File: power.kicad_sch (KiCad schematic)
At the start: 89 parts, among them Q1 PJE138K, Q2 PJE138K, Q3 SSM3J332R, Q4 PJE138K, Q5 SSM3J332R, Q6 PJE138K, Q7 SSM3J332R, U1 TLV70018_SC70, U4 TPS65150_HTSSOP, U5 MPQ7235GQBE, U6 TLV76701_WSON

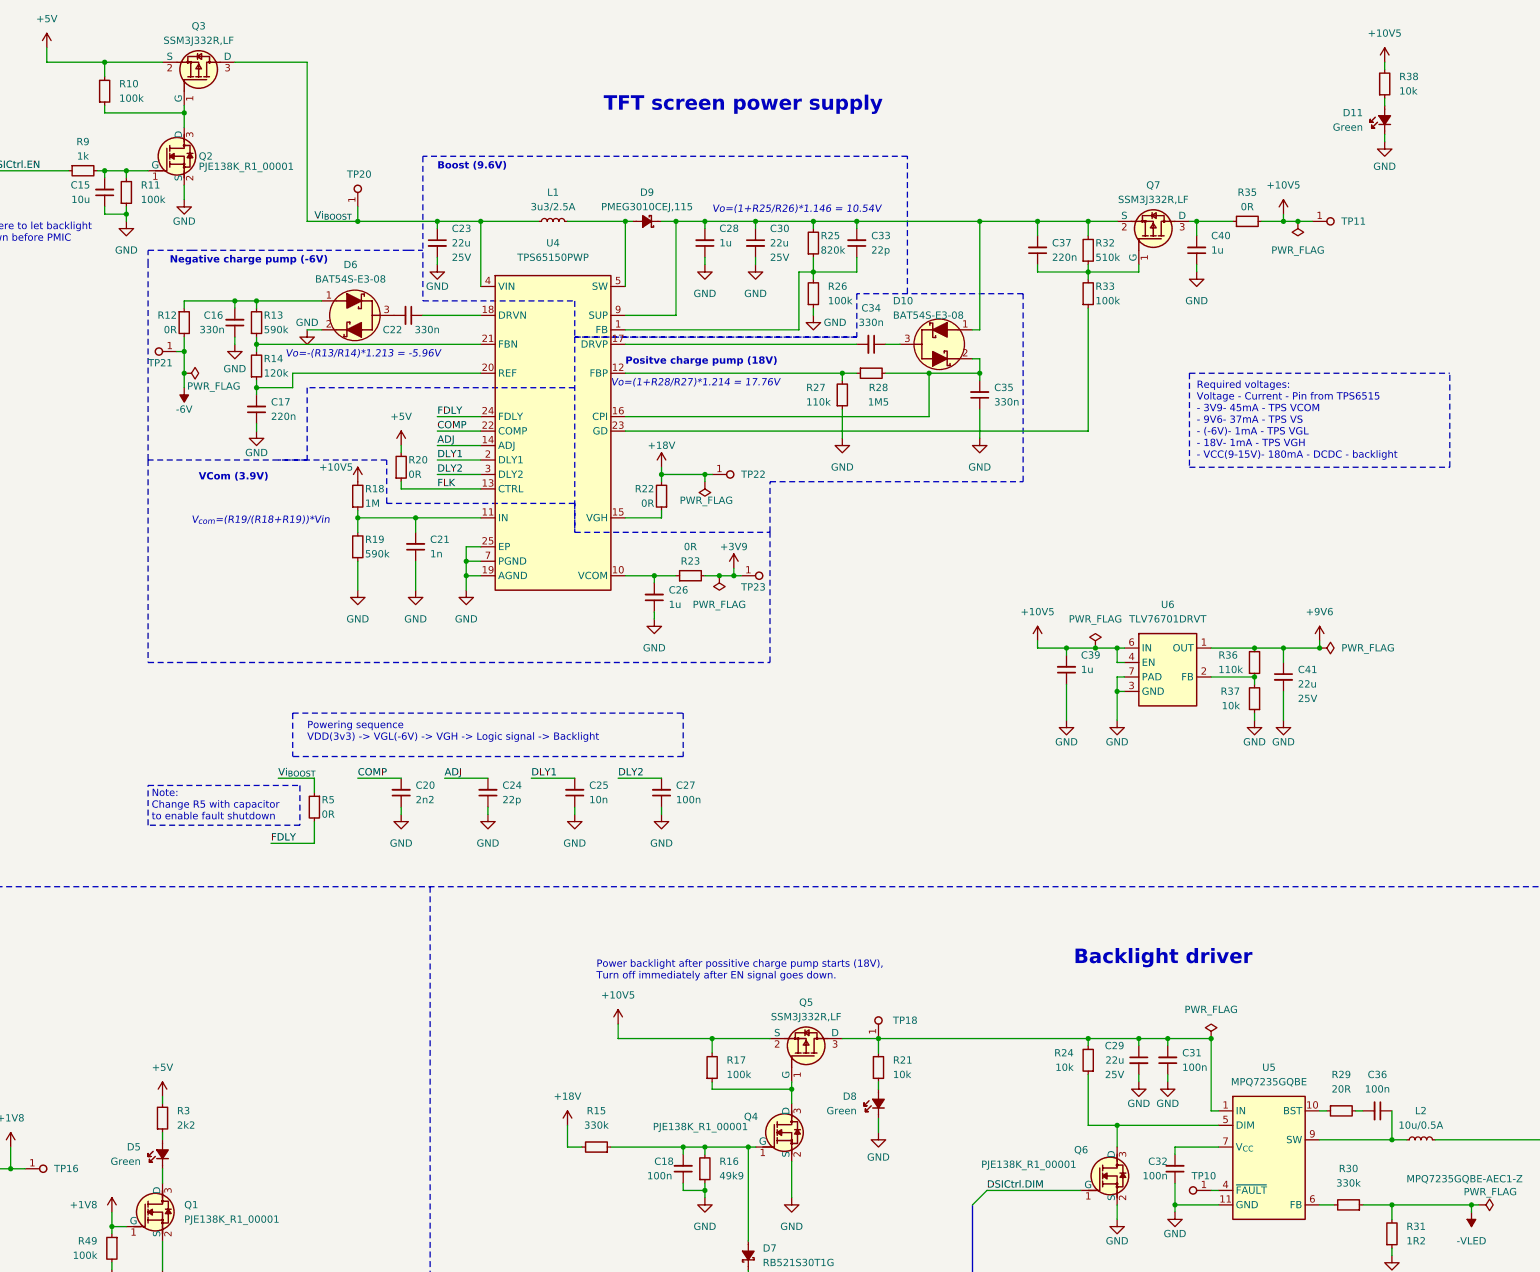
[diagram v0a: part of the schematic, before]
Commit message: [#73840] Change right angle LEDs to vertical (KP-1608ZGC)
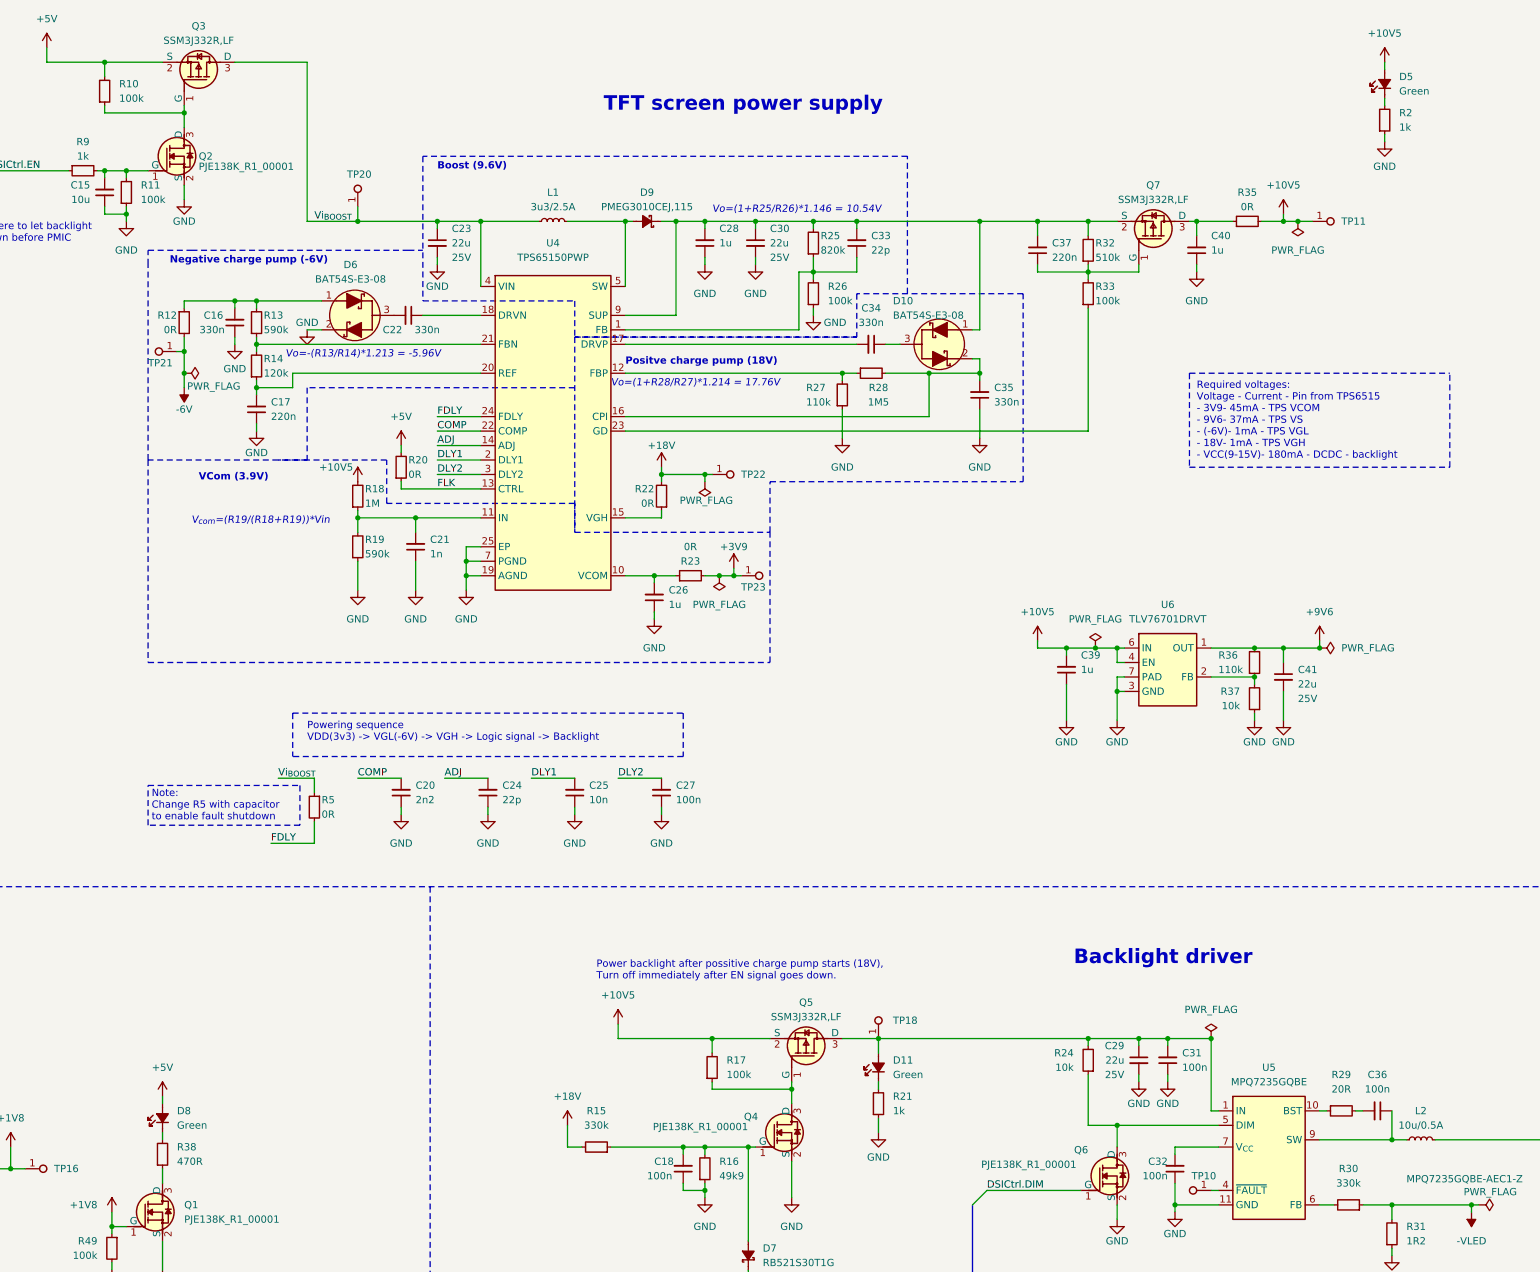
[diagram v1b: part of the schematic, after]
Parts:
- removed D11, D5, D8: LED_G_0603_598-8D80-107F, antmicro-footprints:LED_0603_1608Metric_G_Right_Angle, symbol antmicroLEDIndicationDiscrete:LED_G_0603_598-8D80-107F
- removed R21, R38: R_10k_0402, antmicro-footprints:R_0402_1005Metric, symbol antmicroResistors0402:R_10k_0402
- removed R3: R_2k2_0402, antmicro-footprints:R_0402_1005Metric, symbol antmicroResistors0402:R_2k2_0402
- added D11, D5, D8: LED_G_0603_KP-1608ZGC, antmicro-footprints:LED_0603_1608Metric_G, symbol antmicroLEDIndicationDiscrete:LED_G_0603_KP-1608ZGC
- added R2, R21: R_1k_0402, antmicro-footprints:R_0402_1005Metric, symbol antmicroResistors0402:R_1k_0402
- added R38: R_470R_0402, antmicro-footprints:R_0402_1005Metric, symbol antmicroResistors0402:R_470R_0402
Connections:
- net +10V5: now also D5.2 (A)
- net +5V: now also D8.2 (A)
- net GND: now also R2.1, R21.1
- net at C29.1, C31.2, Q5.3 (D)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: now also D11.2 (A)
- net at Q1.3 (D): now also R38.1
- new net: D8.1 (C), R38.2
- new net: D5.1 (C), R2.2
- new net: D11.1 (C), R21.2
